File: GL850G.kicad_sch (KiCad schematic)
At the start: 54 parts, among them J1 USB_A, J10 Conn_01x02_Pin, J2 USB_A, J3 USB_A, J4 USB_A, J5 USB_A, J6 Conn_01x03_Pin, J7 Conn_01x02_Pin, J8 Conn_01x02_Pin, J9 Conn_01x03_Pin, U1 GL850G, U11 AP2151WG, Y1 12MHz

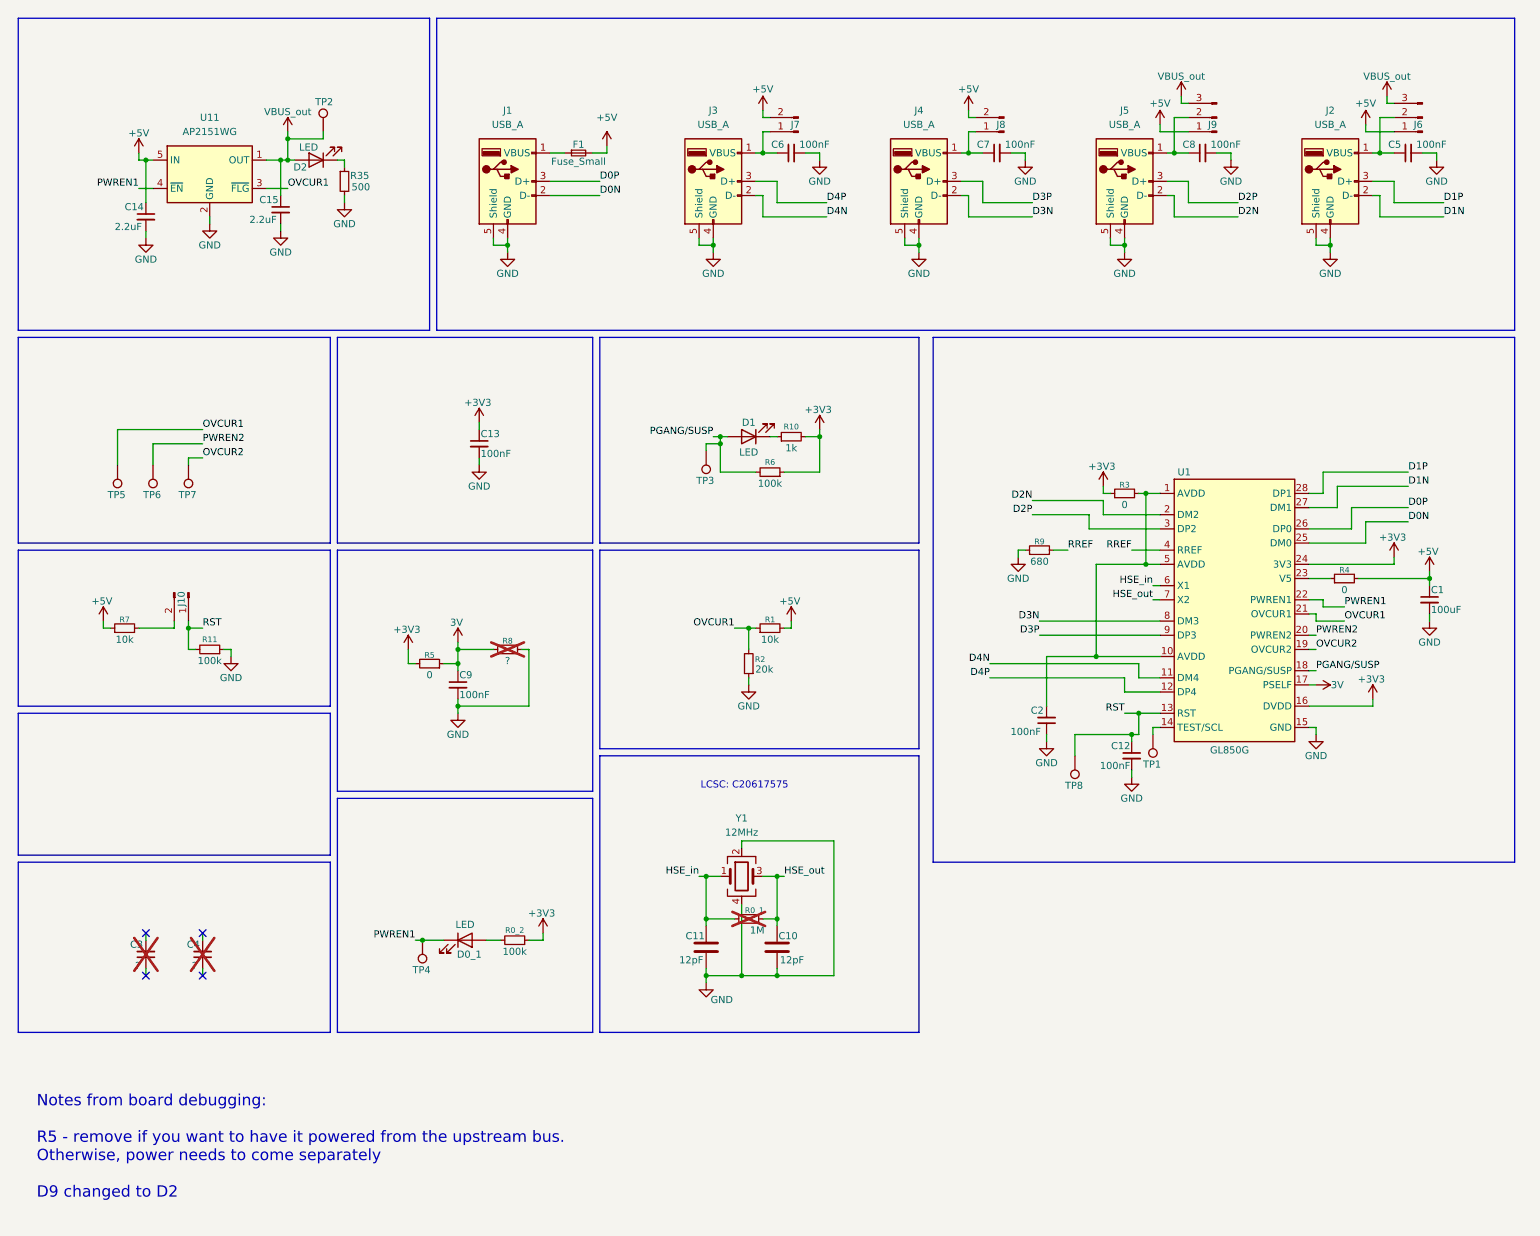
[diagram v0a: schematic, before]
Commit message: modified:   0.My_Library.bak 	modified:   0.My_Library.kicad_sym 	new file:   GL850G-backups/GL850G-2026-01-02_150657.zip 	new file:   GL850G-backups/GL850G-2026-01-02_151627.zip 	new file:   GL850G-backups/GL850G-2026-01-02_160446.zip 	new file:   GL850G-backups/GL850G-2026-01-03_192335.zip 	new file:   GL850G-backups/GL850G-2026-01-03_193700.zip 	new file:   GL850G-backups/GL850G-2026-01-03_194723.zip 	new file:   GL850G-backups/GL850G-2026-01-03_195234.zip 	new file:   GL850G-backups/GL850G-2026-01-03_195824.zip 	modified:   GL850G.kicad_pcb 	modified:   GL850G.kicad_pro 	modified:   GL850G.kicad_sch 	new file:   GL850G_USB_Hub_BACKUP.zip 	modified:   fp-info-cache 	modified:   production/GL850G.zip 	new file:   production/backups/GL850G_2026-01-03_19-52-49.zip 	modified:   production/bom.csv 	modified:   production/designators.csv 	modified:   production/netlist.ipc 	modified:   production/positions.csv
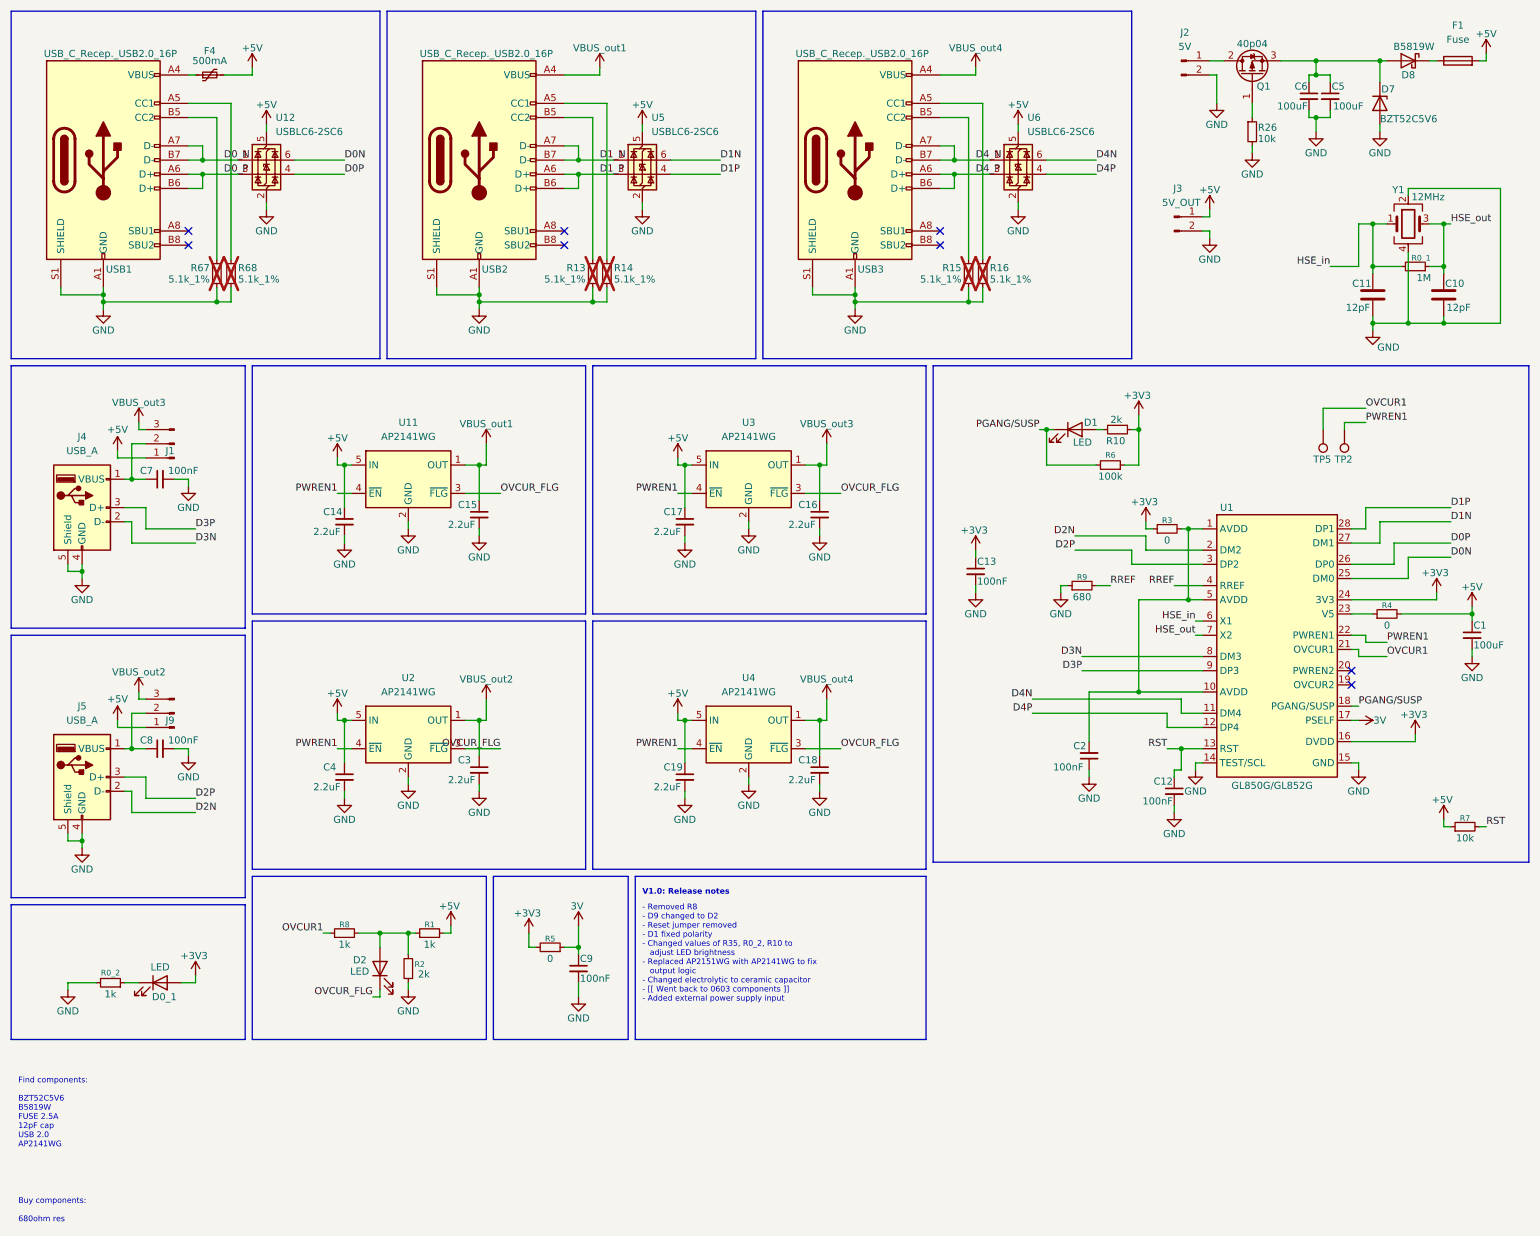
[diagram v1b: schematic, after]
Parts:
- removed F1: Fuse_Small, Fuse:Fuse_1210_3225Metric_Pad1.42x2.65mm_HandSolder, symbol Device:Fuse_Small
- removed J1, J2, J3: USB_A, My_Library:USB_A_2.0, symbol Connector:USB_A
- removed J10, J7, J8: Conn_01x02_Pin, Connector_PinHeader_2.54mm:PinHeader_1x02_P2.54mm_Vertical, symbol Connector:Conn_01x02_Pin
- removed J6: Conn_01x03_Pin, Connector_PinHeader_2.54mm:PinHeader_1x03_P2.54mm_Vertical, symbol Connector:Conn_01x03_Pin
- removed R11: 100k, Resistor_SMD:R_0603_1608Metric_Pad0.98x0.95mm_HandSolder, symbol Device:R_Small
- removed R35: 500, Resistor_SMD:R_0805_2012Metric_Pad1.20x1.40mm_HandSolder, symbol Device:R_Small
- removed TP1, TP3, TP4, TP6, TP7, TP8: TestPoint, TestPoint:TestPoint_Pad_D2.0mm, symbol Connector:TestPoint
- added C16, C17, C18, C19: 2.2uF, Capacitor_SMD:C_0603_1608Metric_Pad1.08x0.95mm_HandSolder, symbol Device:C_Small
- added D7: BZT52C5V6, Diode_SMD:D_SOD-123, symbol Device:D_Zener
- added D8: B5819W, Diode_SMD:D_SOD-123, symbol Device:D_Schottky
- added F1: Fuse, Capacitor_SMD:C_1812_4532Metric_Pad1.57x3.40mm_HandSolder, symbol Device:Fuse
- added F4: 500mA, Fuse:Fuse_0805_2012Metric, symbol Device:Polyfuse_Small
- added J1: Conn_01x03_Pin, Connector_PinHeader_2.54mm:PinHeader_1x03_P2.54mm_Vertical, symbol Connector:Conn_01x03_Pin
- added J2: 5V, Connector_JST:JST_XH_B2B-XH-A_1x02_P2.50mm_Vertical, symbol Connector:Conn_01x02_Pin
- added J3: 5V_OUT, Connector_PinHeader_2.54mm:PinHeader_1x02_P2.54mm_Vertical, symbol Connector:Conn_01x02_Pin
- added Q1: 40p04, Package_TO_SOT_SMD:TO-252-2, symbol Transistor_FET:SUD50P04-08
- added R13, R14, R15, R16, R67, R68: 5.1k_1%, Resistor_SMD:R_0603_1608Metric_Pad0.98x0.95mm_HandSolder, symbol Device:R_Small
- added R26: 10k, Resistor_SMD:R_0603_1608Metric_Pad0.98x0.95mm_HandSolder, symbol Device:R_Small
- added U12, U5, U6: USBLC6-2SC6, Package_TO_SOT_SMD:SOT-23-6, symbol Power_Protection:USBLC6-2SC6
- added U2, U3, U4: AP2141WG, Package_TO_SOT_SMD:SOT-23-5_HandSoldering, symbol Power_Management:AP2161W
- added USB1, USB2, USB3: USB_C_Recep._USB2.0_16P, Connector_USB:USB_C_Receptacle_GCT_USB4105-xx-A_16P_TopMnt_Horizontal, symbol Connector:USB_C_Receptacle_USB2.0_16P
- C1: footprint Capacitor_THT:CP_Radial_D5.0mm_P2.00mm -> Capacitor_SMD:C_1206_3216Metric_Pad1.33x1.80mm_HandSolder
- C3, C4: value ? -> 2.2uF; footprint Capacitor_SMD:C_0805_2012Metric_Pad1.18x1.45mm_HandSolder -> Capacitor_SMD:C_0603_1608Metric_Pad1.08x0.95mm_HandSolder; now fitted; now in the parts list
- C5, C6: value 100nF -> 100uF; footprint Capacitor_SMD:C_0603_1608Metric_Pad1.08x0.95mm_HandSolder -> Capacitor_SMD:C_1206_3216Metric_Pad1.33x1.80mm_HandSolder
- R0_1: now fitted; now in the parts list
- R0_2: value 100k -> 1k
- R1: value 10k -> 1k
- R10: value 1k -> 2k
- R2: value 20k -> 2k
- R8: value ? -> 1k; footprint Capacitor_SMD:C_0805_2012Metric_Pad1.18x1.45mm_HandSolder -> Resistor_SMD:R_0805_2012Metric_Pad1.20x1.40mm_HandSolder; now fitted; now in the parts list
- U1: value GL850G -> GL850G/GL852G
- U11: value AP2151WG -> AP2141WG
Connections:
- net +3V3: now also D0_1.2 (A), R10.1; no longer R0_2.1, R10.2
- net +5V: now also C4.1, C17.1, C19.1, F1.2, F4.2, J1.1 (Pin_1), J3.1 (Pin_1), U12.5 (VBUS), U2.5 (IN), U3.5 (IN), U4.5 (IN), U5.5 (VBUS), U6.5 (VBUS)
- net 3V: no longer R8.1
- net D0N: now also U12.6 (I/O1)
- net D0P: now also U12.4 (I/O2)
- net D1N: now also U5.6 (I/O1)
- net D1P: now also U5.4 (I/O2)
- net D4N: now also U6.6 (I/O1)
- net D4P: now also U6.4 (I/O2)
- net GND: now also C3.2, C4.2, R0_2.2, U1.14 (TEST/SCL), C16.2, C17.2, C18.2, C19.2, D7.2 (A), J2.2 (Pin_2), J3.2 (Pin_2), R13.1, R14.1, R15.1, R16.1, R26.2, R67.1, R68.1, U12.2 (GND), U2.2 (GND), U3.2 (GND), U4.2 (GND), U5.2 (GND), U6.2 (GND), USB1.A1 (GND), USB1.A12 (GND), USB1.B1 (GND), USB1.B12 (GND), USB1.S1 (SHIELD), USB2.A1 (GND), USB2.A12 (GND), USB2.B1 (GND), USB2.B12 (GND), USB2.S1 (SHIELD), USB3.A1 (GND), USB3.A12 (GND), USB3.B1 (GND), USB3.B12 (GND), USB3.S1 (SHIELD); no longer R8.2
- net OVCUR1: now also R8.1; no longer R1.1, R2.2, U11.3 (~{FLG})
- net PGANG/SUSP: now also D1.1 (K); no longer D1.2 (A)
- net PWREN1: now also TP2.1, U2.4 (~{EN}), U3.4 (~{EN}), U4.4 (~{EN}); no longer D0_1.1 (K)
- net RST: now also R7.2
- net at C5.1: now also C6.1, D7.1 (K), D8.2 (A), Q1.3 (S)
- net at C7.1, J4.1 (VBUS): now also J1.2 (Pin_2)
- net OVCUR_FLG: now reaches D2.1 (K)
- net OVCUR_FLG: now also U11.3 (~{FLG}), U2.3 (~{FLG}), U3.3 (~{FLG}), U4.3 (~{FLG})
- net VBUS_out2: now reaches C3.1
- net VBUS_out2: now also J9.3 (Pin_3), U2.1 (OUT)
- net OVCUR2: no longer names the net of U1.19 (OVCUR2)
- net PWREN2: no longer names the net of U1.20 (PWREN2)
- removed net VBUS_out: C15.1, D2.2 (A), J9.3 (Pin_3), TP2.1, U11.1 (OUT)
- new net: D2.2 (A), R1.1, R2.2, R8.2
- new net: D8.1 (K), F1.1
- new net: R15.2, USB3.B5 (CC2)
- new net: D1.2 (A), R10.2
- new net: R68.2, USB1.A5 (CC1)
- new net: R16.2, USB3.A5 (CC1)
- new net: R14.2, USB2.A5 (CC1)
- new net: R13.2, USB2.B5 (CC2)
- new net: F4.1, USB1.A4 (VBUS), USB1.A9 (VBUS), USB1.B4 (VBUS), USB1.B9 (VBUS)
- new net: R67.2, USB1.B5 (CC2)
- new net: D0_1.1 (K), R0_2.1
- new net: J2.1 (Pin_1), Q1.2 (D)
- new net: Q1.1 (G), R26.1
- new net D0_N: U12.1 (I/O1), USB1.A7 (D-), USB1.B7 (D-)
- new net D0_P: U12.3 (I/O2), USB1.A6 (D+), USB1.B6 (D+)
- new net D1_N: U5.1 (I/O1), USB2.A7 (D-), USB2.B7 (D-)
- new net D1_P: U5.3 (I/O2), USB2.A6 (D+), USB2.B6 (D+)
- new net D4_N: U6.1 (I/O1), USB3.A7 (D-), USB3.B7 (D-)
- new net D4_P: U6.3 (I/O2), USB3.A6 (D+), USB3.B6 (D+)
- new net VBUS_out1: C15.1, U11.1 (OUT), USB2.A4 (VBUS), USB2.A9 (VBUS), USB2.B4 (VBUS), USB2.B9 (VBUS)
- new net VBUS_out3: C16.1, J1.3 (Pin_3), U3.1 (OUT)
- new net VBUS_out4: C18.1, U4.1 (OUT), USB3.A4 (VBUS), USB3.A9 (VBUS), USB3.B4 (VBUS), USB3.B9 (VBUS)
- no-connect marks 4 -> 8
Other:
- note added: "- Removed R8 - D9 changed to D2 - Reset jumper removed - D1 fixed polarity - Changed values of R35, R0_2, R10 to adjust LED brightness - Replaced AP2151WG with AP2141WG to fix output logic - Changed electrolytic to ceramic capacitor - [[ Went back to 0603 components ]] - Added external power supply input"
- note added: "Buy components: 680ohm res"
- note added: "Find components: BZT52C5V6 B5819W FUSE 2.5A 12pF cap USB 2.0 AP2141WG"
- note added: "V1.0: Release notes"
- note removed: "LCSC: C20617575"
- note removed: "Notes from board debugging: R5 - remove if you want to have it powered from the upstream bus. Otherwise, power needs to come separately D9 changed to D2"
- moved on the sheet: C1, C10, C11, C12, C13, C14, C15, C2, C7, C8, C9, D0_1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
